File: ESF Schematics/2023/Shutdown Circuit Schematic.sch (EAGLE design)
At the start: 67 parts, among them J1 CONNECTOR-1_LCAX2-14F-E, J2 CONNECTOR-1_LCAX2-14F-E, J3 CONNECTOR-1_LCAX2-14F-E, J4 CONNECTOR-1_LCAX2-14F-E, Q1 MOSFET_N-CHANNEL, Q2 MOSFET_N-CHANNEL, U1 LOGICGATE_INVERTER, U2 LOGICGATE_INVERTER

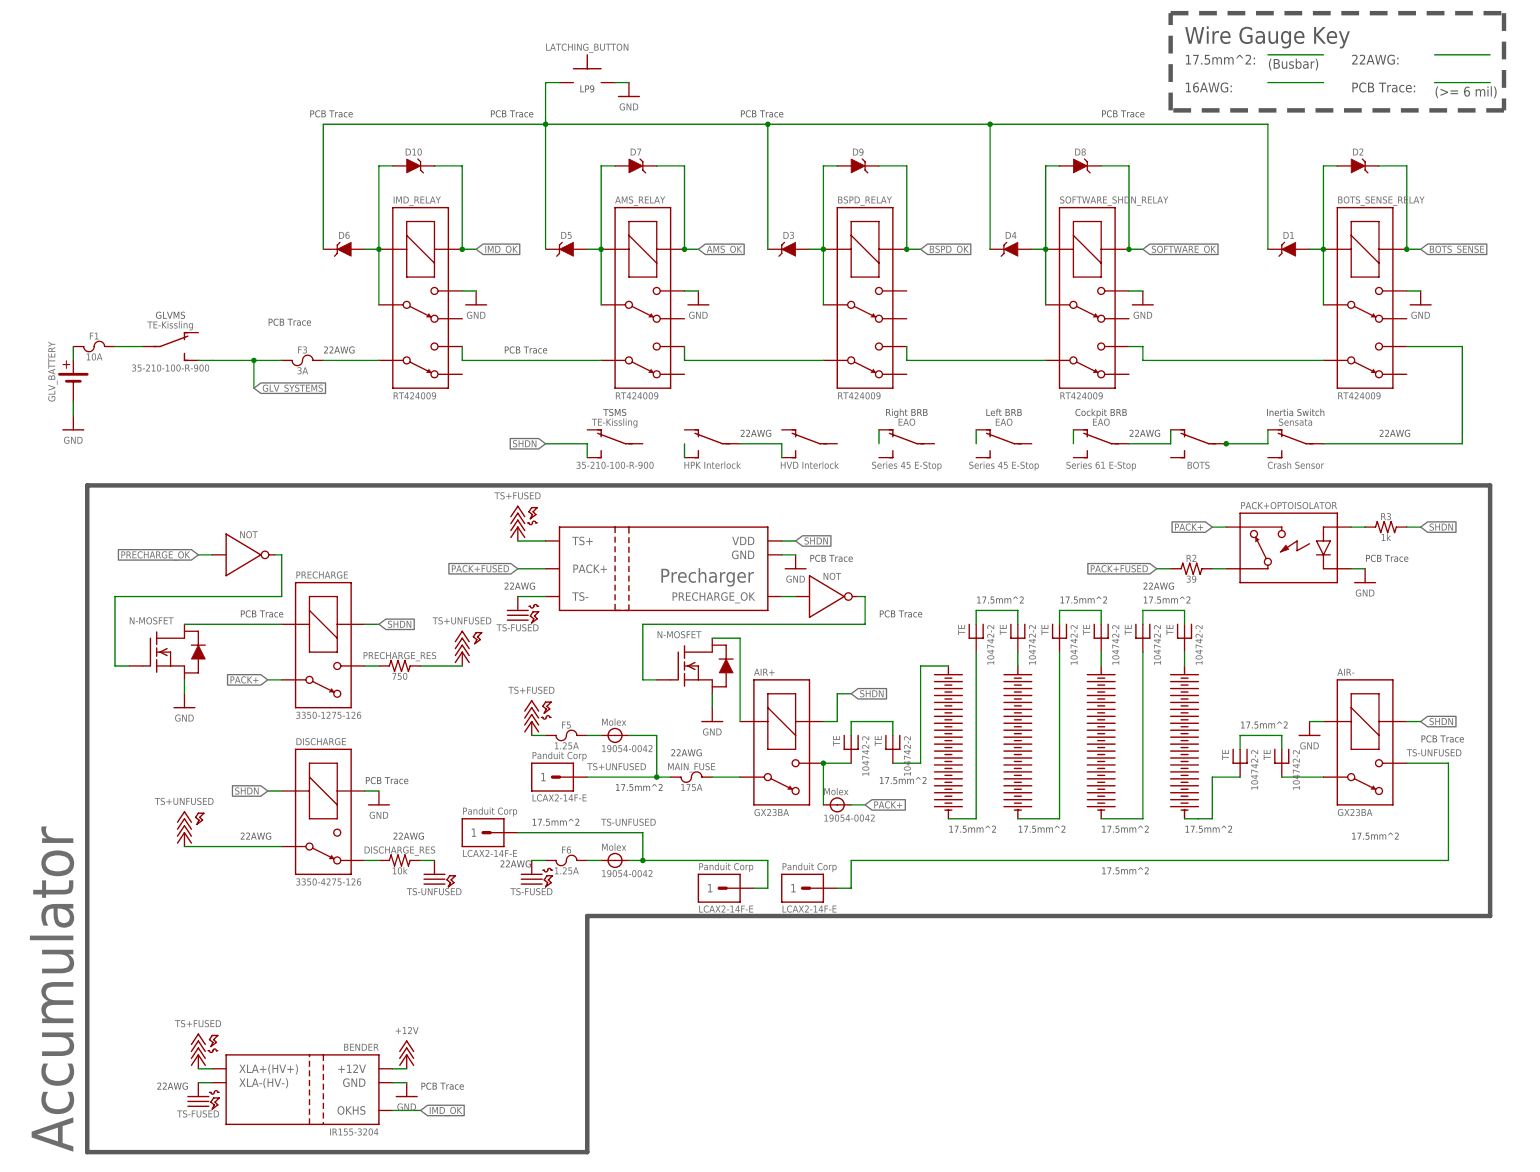
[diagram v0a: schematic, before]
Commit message: more work done
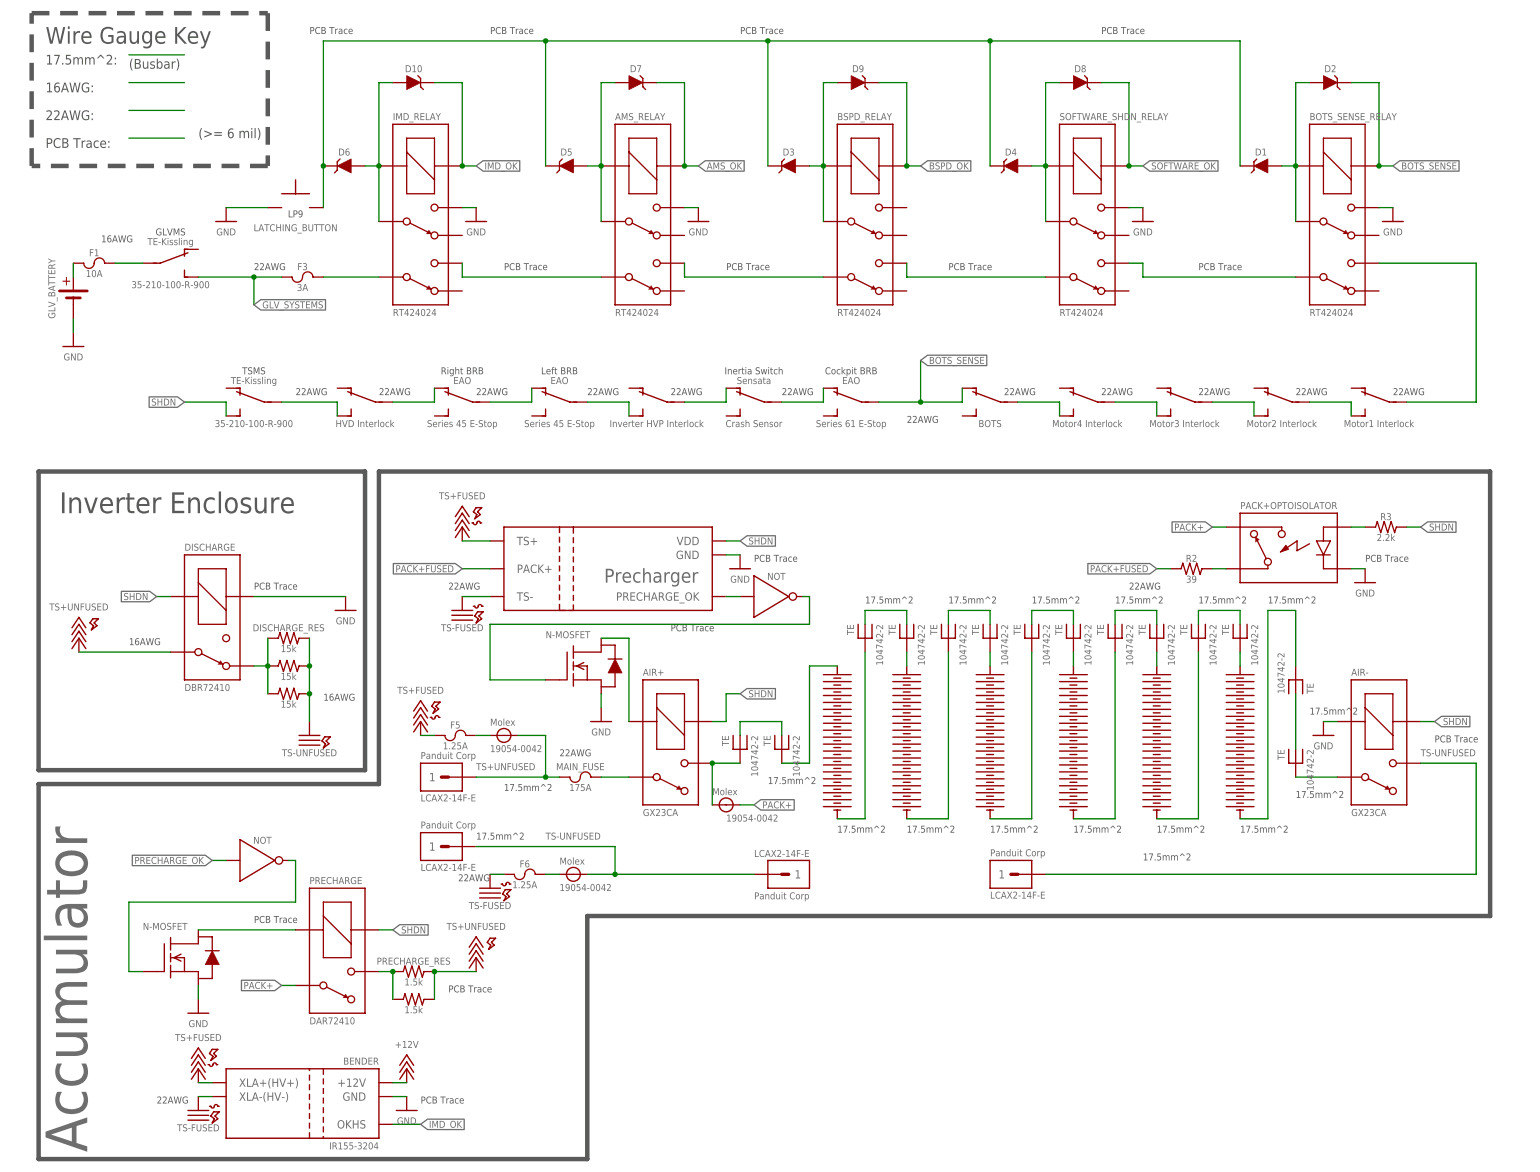
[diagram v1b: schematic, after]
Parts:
- added DISCHARGE_RES1, DISCHARGE_RES2: 15k, HyTechSymbolsTemp:RESISTOR
- added PRECHARGE_RES1: 1.5k, HyTechSymbolsTemp:RESISTOR
- added S10, S11, S12, S13: SWITCH_SPST_, HyTechSymbols:SWITCH_SPST_
- added U$1, U$4: SEGMENT, HyTechSymbols:SEGMENT
- added U$2, U$3, U$5, U$6: MAINTENANCE_PLUG_104742-2, HyTechSymbolsTemp:MAINTENANCE_PLUG_104742-2
- AIR+, AIR-: value RELAY_SPST_NO_GX23BA -> RELAY_SPST_NO_; device HyTechSymbolsTemp:RELAY_SPST_NO_GX23BA -> HyTechSymbols:RELAY_SPST_NO_; MPN (none) -> GX23CA
- AMS_RELAY, BOTS_SENSE_RELAY, BSPD_RELAY, IMD_RELAY, SOFTWARE_SHDN_RELAY: value RELAY_DPDT_RT424009 -> RELAY_DPDT_RT424024; device HyTechSymbolsTemp:RELAY_DPDT_RT424009 -> HyTechSymbols:RELAY_DPDT_RT424024
- DISCHARGE: value RELAY_SPST_NC_3350-4275-126 -> RELAY_SPST_NC_DBR72410; device HyTechSymbolsTemp:RELAY_SPST_NC_3350-4275-126 -> HyTechSymbols:RELAY_SPST_NC_DBR72410
- DISCHARGE_RES: value 10k -> 15k
- PRECHARGE: value RELAY_SPST_NO_3350-1275-126 -> RELAY_SPST_NO_DAR72410; device HyTechSymbolsTemp:RELAY_SPST_NO_3350-1275-126 -> HyTechSymbols:RELAY_SPST_NO_DAR72410
- PRECHARGE_RES: value 750 -> 1.5k
- R3: value 1k -> 2.2k
- S7: MPN HPK Interlock -> Inverter HVP Interlock
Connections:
- new net N$17: S12.P, S13.S
- new net N$18: S11.P, S12.S
- new net N$20: S10.P, S11.S
- new net N$30: S10.S, S2.P
- new net N$54: U$1.+, U$3.1
- new net N$55: U$2.P$1, U$3.P$1
- new net N$56: U$36.1, U$4.-
- new net N$57: U$4.+, U$6.1
- new net N$58: U$5.P$1, U$6.P$1
- net BOTS_SENSE: now also S2.O, S3.P
- net GND: now also LATCHING_BUTTON.P$1; no longer LATCHING_BUTTON.P$2
- net N$12: now also S5.P
- net N$13: now also S6.P
- net N$19: now also S13.P; no longer S1.P
- net N$2: now also LATCHING_BUTTON.P$2; no longer LATCHING_BUTTON.P$1
- net N$21: now also S8.P; no longer S7.P
- net N$23: now also U$1.-, U$5.1; no longer U$15.-, U$36.1
- net N$26: now also PRECHARGE_RES1.1
- net N$29: now also DISCHARGE_RES1.1, DISCHARGE_RES2.1
- net N$4: now also S7.P; no longer S2.P
- net N$51: now also S4.P
- net N$8: now also S1.P
- net N$9: now also U$15.-, U$2.1; no longer S2.O, S3.P
- net TS+UNFUSED: now also PRECHARGE_RES1.2
- net TS-UNFUSED: now also DISCHARGE_RES1.2, DISCHARGE_RES2.2
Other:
- note added: "16AWG"
- note added: "Inverter Enclosure"
- moved on the sheet: AIR+, AIR-, AMS_RELAY, BOTS_SENSE_RELAY, BSPD_RELAY, D1, D10, D2, D3, D4, D5, D6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
